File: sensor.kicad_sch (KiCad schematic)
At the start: 139 parts, among them U1 Hall_Sensor, U10 Hall_Sensor, U11 Hall_Sensor, U12 Hall_Sensor, U13 Hall_Sensor, U14 Hall_Sensor, U15 Hall_Sensor, U16 Hall_Sensor, U17 Hall_Sensor, U18 Hall_Sensor, U19 Hall_Sensor, U2 Hall_Sensor, U20 Hall_Sensor, U21 Hall_Sensor, U22 Hall_Sensor, U23 Hall_Sensor, U24 Hall_Sensor, U25 Hall_Sensor, U26 Hall_Sensor, U27 Hall_Sensor, U28 Hall_Sensor, U29 Hall_Sensor, U3 Hall_Sensor, U30 Hall_Sensor, U31 Hall_Sensor, U32 Hall_Sensor, U33 Hall_Sensor, U34 Hall_Sensor, U35 Hall_Sensor, U36 Hall_Sensor, U37 Hall_Sensor, U38 Hall_Sensor, U39 Hall_Sensor, U4 Hall_Sensor, U40 Hall_Sensor, U41 Hall_Sensor, U42 Hall_Sensor, U43 Hall_Sensor, U44 Hall_Sensor, U45 Hall_Sensor, U46 Hall_Sensor, U47 Hall_Sensor, U48 Hall_Sensor, U49 Hall_Sensor, U5 Hall_Sensor, U50 Hall_Sensor, U51 Hall_Sensor, U52 Hall_Sensor, U53 Hall_Sensor, U54 Hall_Sensor, U55 Hall_Sensor, U56 Hall_Sensor, U57 Hall_Sensor, U58 Hall_Sensor, U59 Hall_Sensor, U6 Hall_Sensor, U60 Hall_Sensor, U61 Hall_Sensor, U62 Hall_Sensor, U63 Hall_Sensor, U64 Hall_Sensor, U65 Hall_Sensor, U66 Hall_Sensor, U7 Hall_Sensor, U8 Hall_Sensor, U9 Hall_Sensor

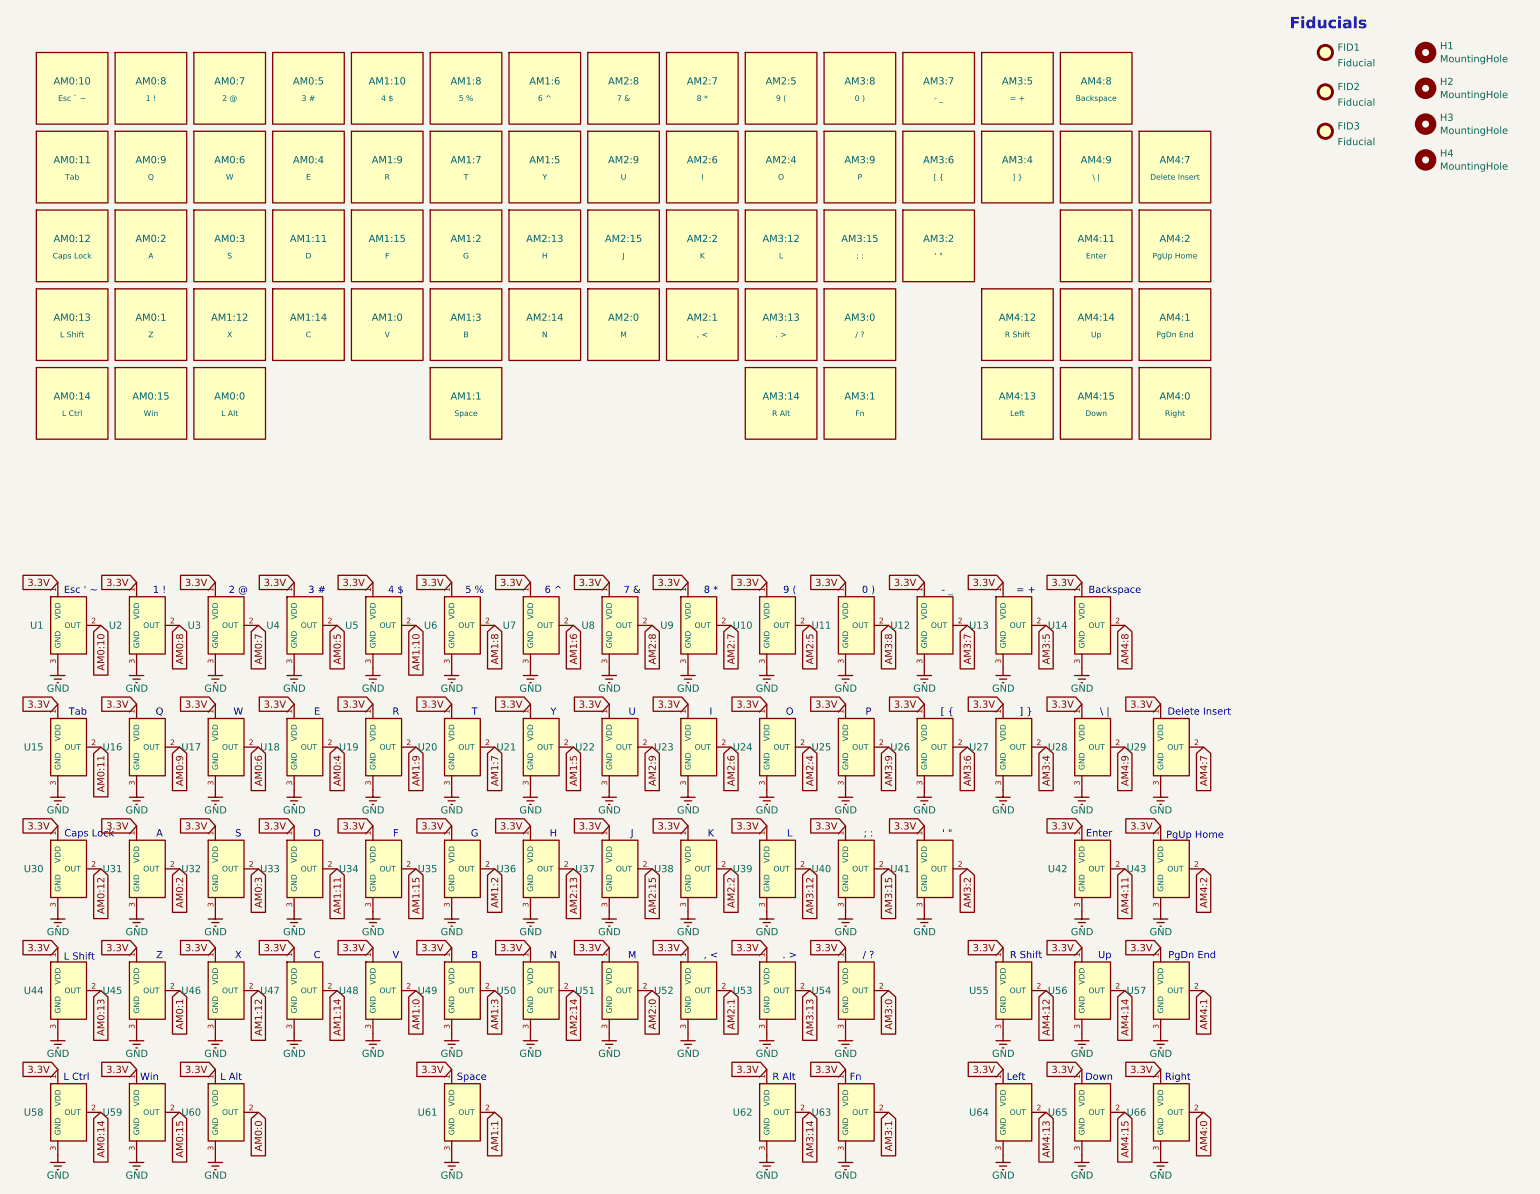
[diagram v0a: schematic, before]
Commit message: Sixth Commit
Almost done. Just need to make sure the field zone and each pin is connected properly
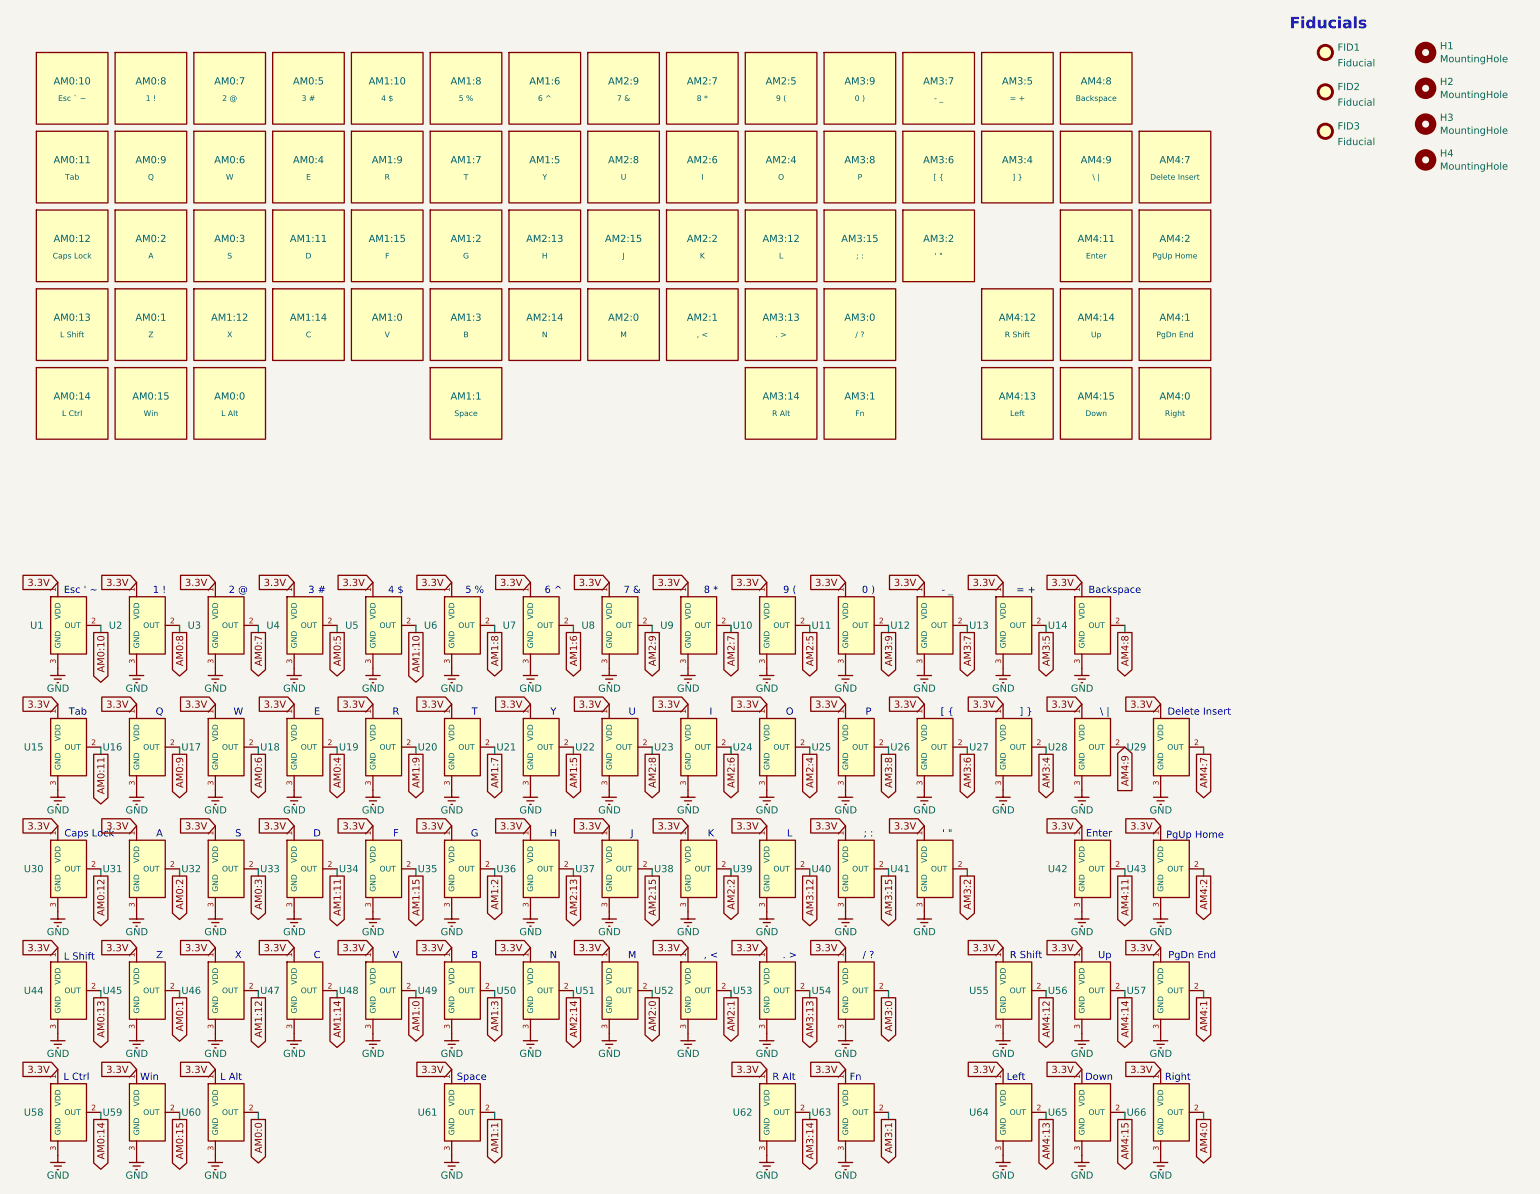
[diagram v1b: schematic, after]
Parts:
- renumbered AM2:9 to AM2:8, AM2:8 to AM2:9, AM3:9 to AM3:8, AM3:8 to AM3:9
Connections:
- net AM2:8: now also U22.2 (OUT); no longer U8.2 (OUT)
- net AM2:9: now also U8.2 (OUT); no longer U22.2 (OUT)
- net AM3:8: now also U25.2 (OUT); no longer U11.2 (OUT)
- net AM3:9: now also U11.2 (OUT); no longer U25.2 (OUT)
